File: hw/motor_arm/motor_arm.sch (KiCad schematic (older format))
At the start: 52 parts, among them J1 Conn_01x05, U1 AP7370-33W5-7, U10 RF4E110GN, U11 RF4E110GN, U2 IR2101, U3 RF4E110GN, U4 RF4E110GN, U5 IR2101, U6 RF4E110GN, U7 EFM8BB21F16I-C-QFN20, U8 RF4E110GN, U9 IR2101

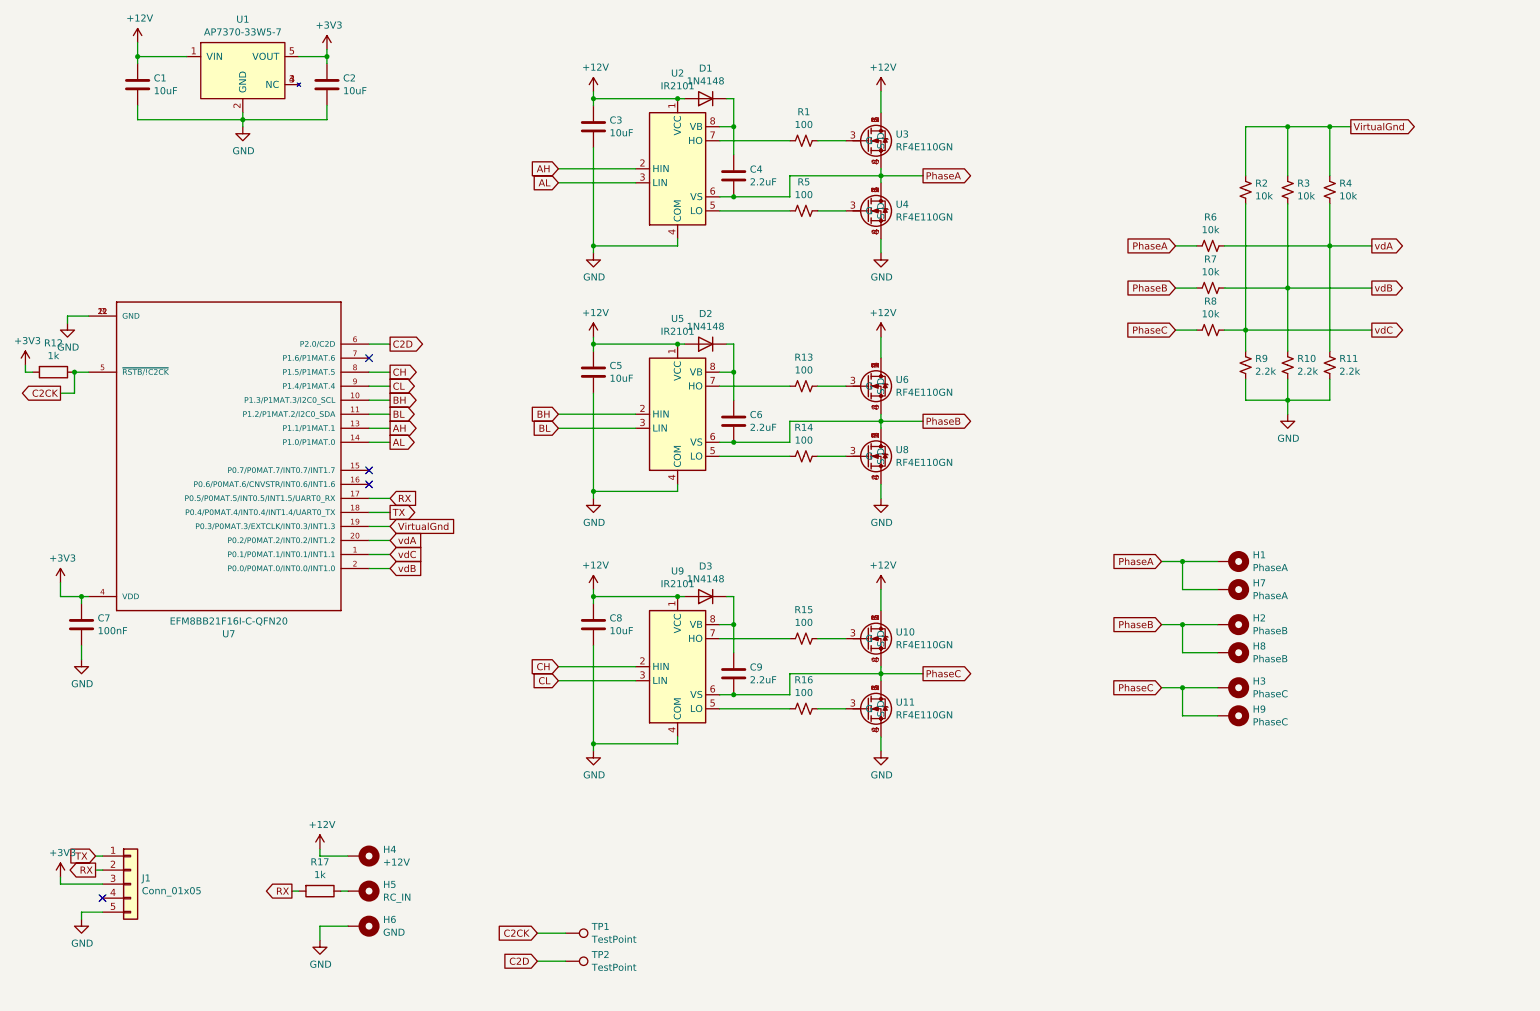
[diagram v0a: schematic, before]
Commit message: created test pcb
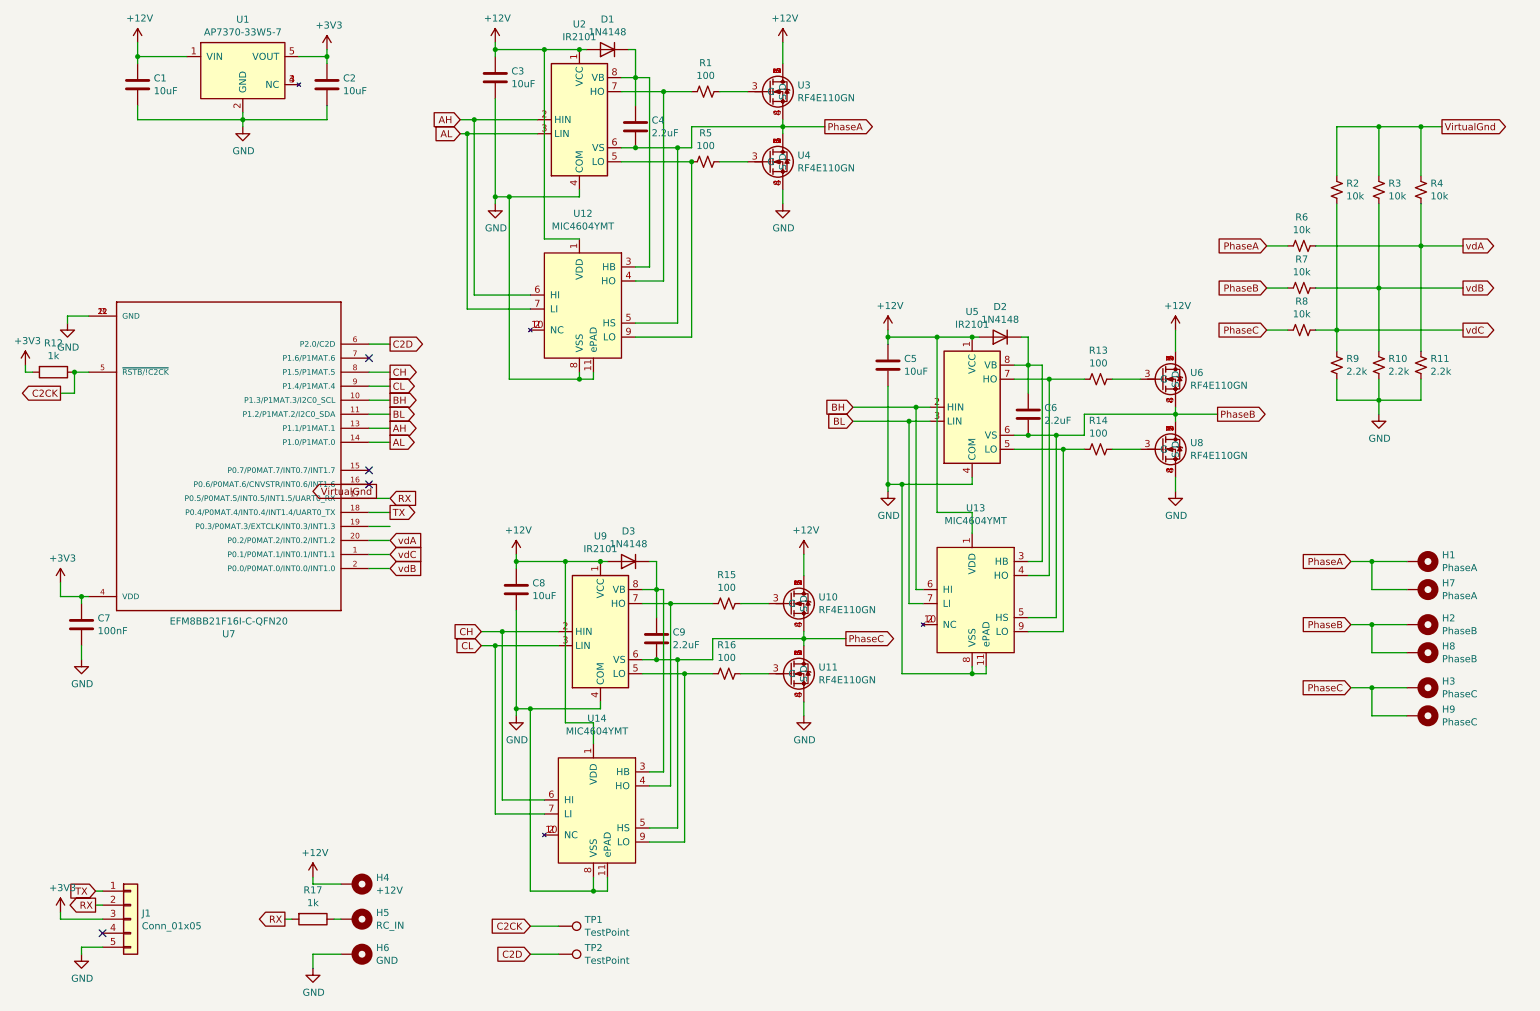
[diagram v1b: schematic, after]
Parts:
- added U12, U13, U14: MIC4604YMT, Custom:MIC4604-TDFN2525-10, symbol Custom:MIC4604YMT
- C1, C2, C3, C4, C5, C6, C7, C8, C9: footprint Capacitor_SMD:C_0805_2012Metric_Pad1.15x1.40mm_HandSolder -> Capacitor_SMD:C_0603_1608Metric_Pad1.05x0.95mm_HandSolder
- R1, R10, R11, R12, R13, R14, R15, R16, R17, R2, R3, R4, R5, R6, R7, R8, R9: footprint Resistor_SMD:R_0805_2012Metric_Pad1.15x1.40mm_HandSolder -> Resistor_SMD:R_0603_1608Metric_Pad1.05x0.95mm_HandSolder
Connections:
- net +12V: now also U12.1 (VDD), U13.1 (VDD), U14.1 (VDD)
- net AH: now also U12.6 (HI)
- net AL: now also U12.7 (LI)
- net BH: now also U13.6 (HI)
- net BL: now also U13.7 (LI)
- net CH: now also U14.6 (HI)
- net CL: now also U14.7 (LI)
- net GND: now also U12.11 (ePAD), U12.8 (VSS), U13.11 (ePAD), U13.8 (VSS), U14.11 (ePAD), U14.8 (VSS)
- net PhaseA: now also U12.5 (HS)
- net PhaseB: now also U13.5 (HS)
- net PhaseC: now also U14.5 (HS)
- net VirtualGnd: no longer U7.19 (P0.3/P0MAT.3/EXTCLK/INT0.3/INT1.3)
- net at R5.2, U2.5 (LO): now also U12.9 (LO)
- net at R1.2, U2.7 (HO): now also U12.4 (HO)
- net at C4.1, D1.1 (K), U2.8 (VB): now also U12.3 (HB)
- net at R14.2, U5.5 (LO): now also U13.9 (LO)
- net at R13.2, U5.7 (HO): now also U13.4 (HO)
- net at C6.1, D2.1 (K), U5.8 (VB): now also U13.3 (HB)
- net at R16.2, U9.5 (LO): now also U14.9 (LO)
- net at R15.2, U9.7 (HO): now also U14.4 (HO)
- net at C9.1, D3.1 (K), U9.8 (VB): now also U14.3 (HB)
- new net: U12.10 (NC), U12.2 (NC)
- new net: U13.10 (NC), U13.2 (NC)
- new net: U14.10 (NC), U14.2 (NC)
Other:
- moved on the sheet: C3, C4, C5, C6, C8, C9, D1, D2, D3, H1, H2, H3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

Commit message: Update repo with latest local
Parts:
- U1: symbol Custom:AP7370-33W5-7 -> motor_arm-rescue:AP7370-33W5-7-Custom
- U12, U13, U14: symbol Custom:MIC4604YMT -> motor_arm-rescue:MIC4604YMT-Custom
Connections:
- net VirtualGnd: now also U7.19 (P0.3/P0MAT.3/EXTCLK/INT0.3/INT1.3)
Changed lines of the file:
@@
 	10550 2300 10850 2300
 $Comp
-L Custom:AP7370-33W5-7 U1
+L motor_arm-rescue:AP7370-33W5-7-Custom U1
 U 1 1 5EBE3C3B
 P 2150 1050
@@
 Text GLabel 3200 4500 2    50   Input ~ 0
 vdC
-Text GLabel 2650 4050 2    50   Input ~ 0
+Text GLabel 3200 4300 2    50   Input ~ 0
 VirtualGnd
 Wire Wire Line
@@
 	5550 1200 5750 1200
 $Comp
-L Custom:MIC4604YMT U12
+L motor_arm-rescue:MIC4604YMT-Custom U12
 U 1 1 5EC14DDB
 P 4550 2700
@@
 $EndComp
 $Comp
-L Custom:MIC4604YMT U13
+L motor_arm-rescue:MIC4604YMT-Custom U13
 U 1 1 5EC156C7
 P 7350 4800
@@
 $EndComp
 $Comp
-L Custom:MIC4604YMT U14
+L motor_arm-rescue:MIC4604YMT-Custom U14
 U 1 1 5EC252BD
 P 4650 6300
